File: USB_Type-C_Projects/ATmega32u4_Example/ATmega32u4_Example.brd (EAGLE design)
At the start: 9.2 x 7.2 mm, 52 parts, among them J1 105450-0101, J2 282834-3, J3 282834-3, J4 MF-CON-2.54mm-01x11, J5 MF-CON-2.54mm-01x11, SW1 MF-SW-TACT-4.2MM, SW2 MF-SW-TACT-4.2MM, SW3 MF-SW-TACT-4.2MM, SW4 MF-SW-TACT-4.2MM, SW5 MF-SW-TACT-4.2MM, U1 IP4234CZ6,125, U2 ATMEGA32U4-AU, X1 ABM3B-16.000MHZ-D-1-X-T

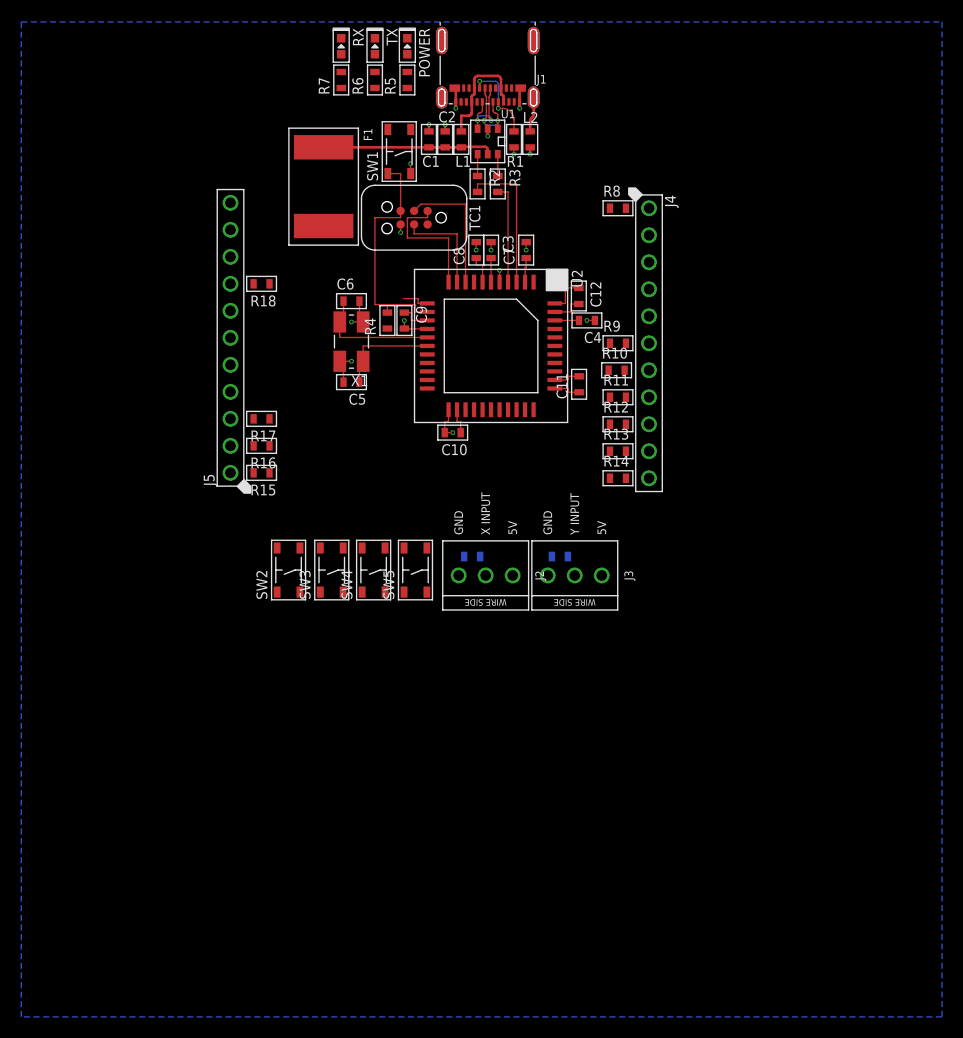
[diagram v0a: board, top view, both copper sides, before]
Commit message: Routing complete
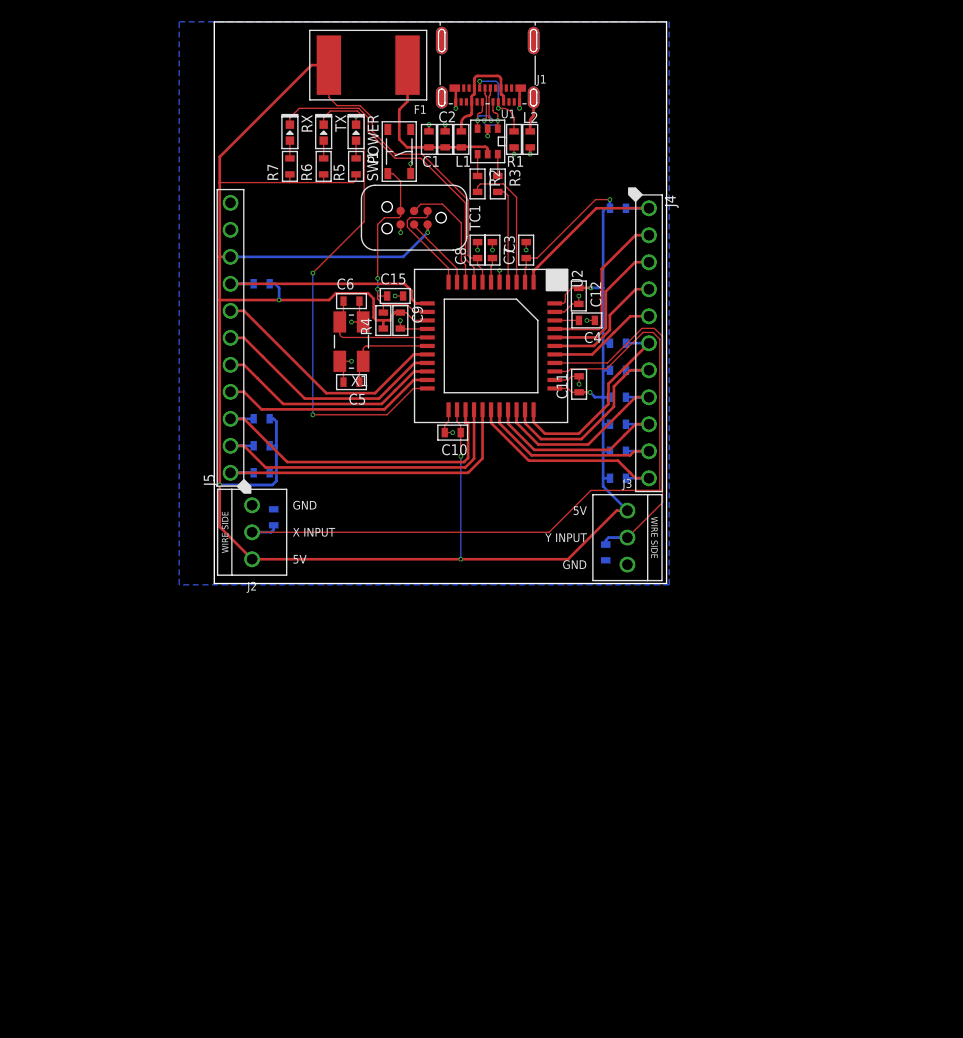
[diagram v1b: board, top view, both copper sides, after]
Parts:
- removed SW2, SW3, SW4, SW5: MF-SW-TACT-4.2MM, MF_Switches:TACT4.2MM
- added C15: 0.1uF, MF_Passives:C0603
- moved J2 22.3 mm to (-7.24, 13.5), turned to 90 degrees
- moved C13 19.0 mm to (-5.21, 14.9), turned to 90 degrees
- moved F1 12.2 mm to (3.68, 57.4), turned to 180 degrees
- moved POWER 9.45 mm to (2.54, 51.1)
- moved R5 9.45 mm to (2.54, 47.9)
- moved R6 9.45 mm to (-0.51, 47.9)
- moved R7 9.45 mm to (-3.68, 47.9)
- moved RX 9.45 mm to (-3.68, 51.1)
- moved TX 9.45 mm to (-0.51, 51.1)
- moved J3 6.10 mm to (28.1, 13.0), turned to 270 degrees
- moved C14 4.33 mm to (26.0, 11.6), turned to 270 degrees
- moved C9 0.38 mm to (6.71, 33.4)
- moved R4 0.38 mm to (5.11, 33.4)
- moved R10 0.13 mm to (27.2, 28.7), flipped to the bottom, turned to 180 degrees
- moved C3 0.13 mm to (15.4, 40.0)
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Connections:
- net 5V: now also R6.P$1, R7.P$1
- net D4: no longer SW2.P$1, SW2.P$2
- net D5*: no longer SW3.P$1, SW3.P$2
- net D6*: no longer SW4.P$1, SW4.P$2
- net D7: no longer SW5.P$1, SW5.P$2
- net GND: now also C15.P$2, J5.P$11; no longer RX.CATHODE, SW2.P$3, SW2.P$4, SW3.P$3, SW3.P$4, SW4.P$3, SW4.P$4, SW5.P$3, SW5.P$4, TX.CATHODE
- net RESET: now also C15.P$1
- net RXLED: now also RX.CATHODE; no longer R7.P$1
- net TXLED: now also TX.CATHODE; no longer R6.P$1
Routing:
- net 5V: track 17.0 -> 267.3 mm, vias 0 -> 8
- net A0: track 0.00 -> 68.4 mm
- net TXLED: track 0.00 -> 46.7 mm, vias 0 -> 2
- net A1: track 0.00 -> 34.6 mm
- net D4: track 0.00 -> 31.1 mm
- net D6*: track 0.00 -> 31.0 mm
- net IO12: track 0.00 -> 30.9 mm
- net RXLED: track 0.00 -> 29.8 mm
- net D3/SCL: track 0.00 -> 23.2 mm
- net D2/SDA: track 0.00 -> 22.3 mm
- net D0/RX: track 0.00 -> 21.3 mm
- net IO8: track 0.00 -> 20.4 mm
- net D1/TX: track 0.00 -> 20.3 mm
- net IO13*: track 0.00 -> 19.5 mm
- net HWB: track 0.00 -> 19.3 mm
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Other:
- board size 9.2 x 7.2 mm -> 42.5 x 52.8 mm

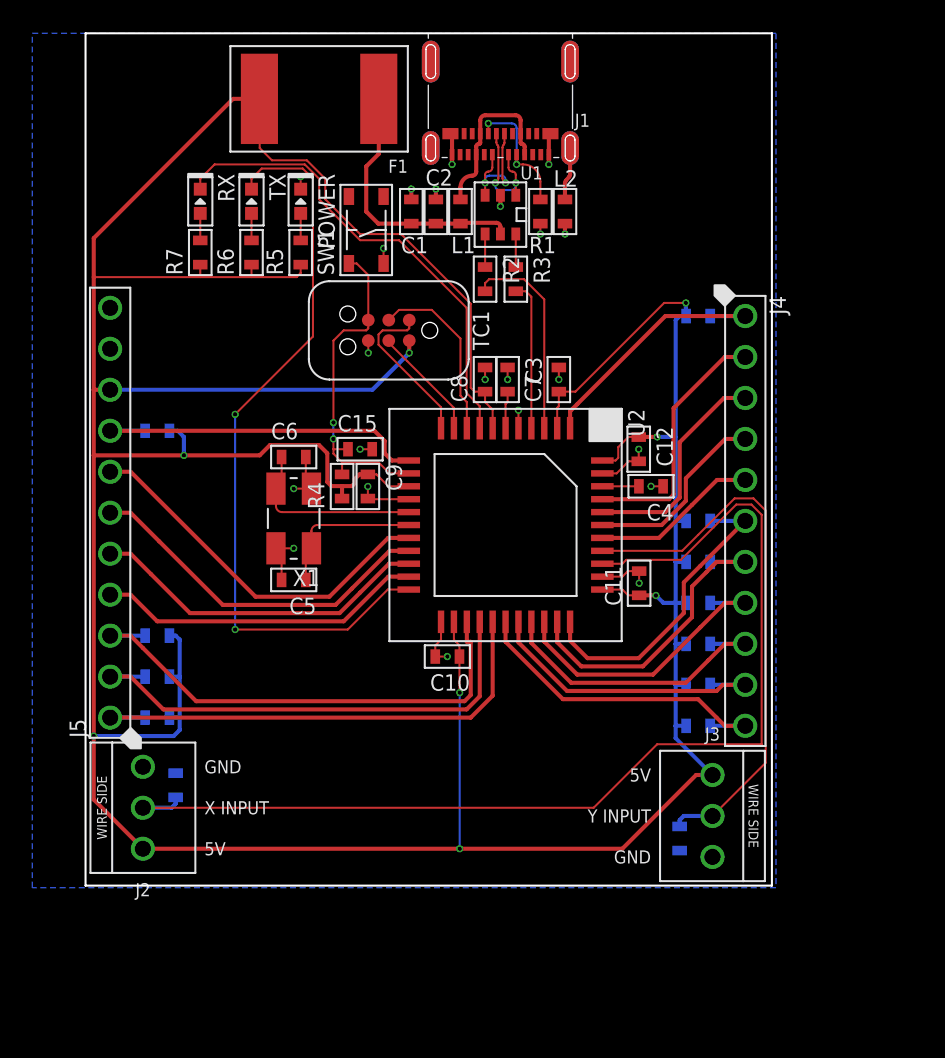
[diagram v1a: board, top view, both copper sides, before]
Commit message: PCB complete. First rev ordered.
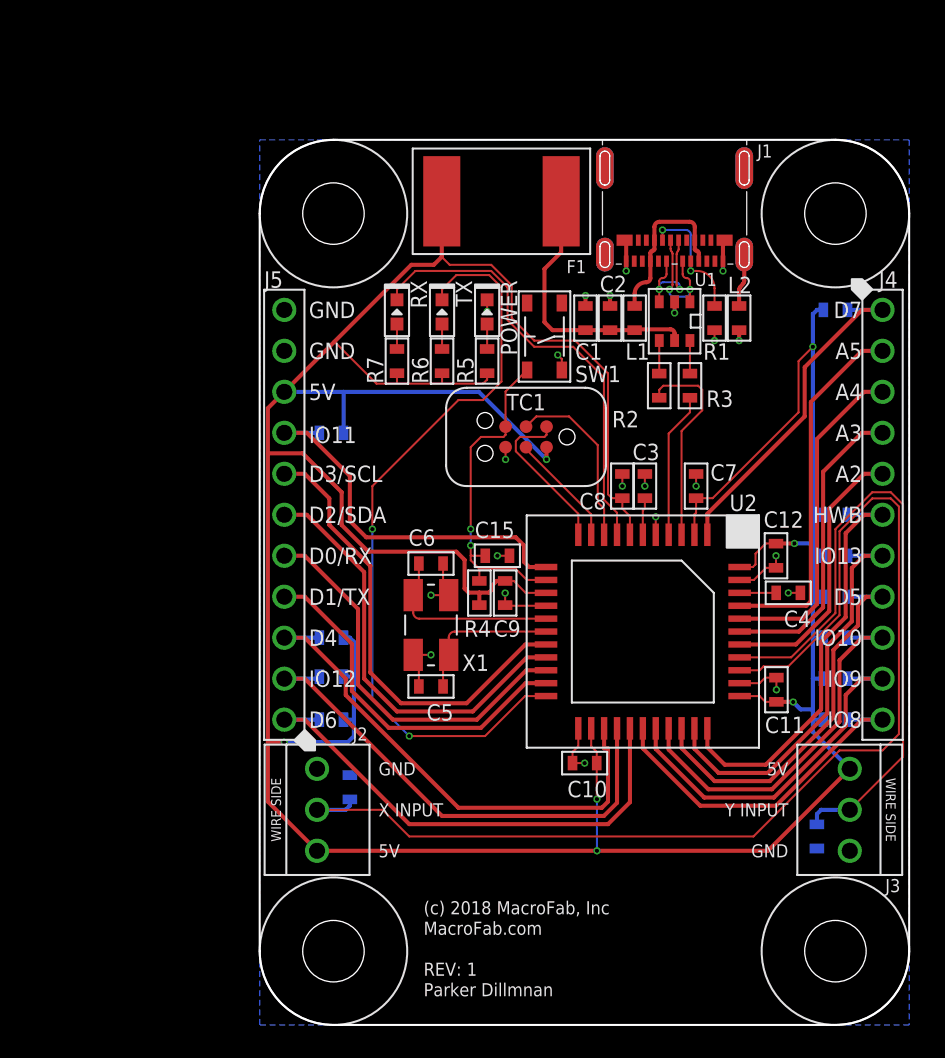
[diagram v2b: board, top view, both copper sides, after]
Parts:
- added FRAME1: MF_FRAMEDEFAULT, MF_Aesthetics:MF_FRAME_DEFAULT
- added H1, H2, H3, H4: MOUNT_HOLE150MIL, PP_Connectors:MOUNT_HOLE_150MIL
- moved RX 14.0 mm to (8.51, 44.2)
- moved R7 13.9 mm to (8.51, 41.1)
- moved TX 13.7 mm to (11.3, 44.2)
- moved R6 13.6 mm to (11.3, 41.1)
- moved POWER 13.4 mm to (14.1, 44.2)
- moved R5 13.4 mm to (14.1, 41.1)
- moved F1 13.0 mm to (15.0, 51.1)
- moved SW1 12.9 mm to (17.7, 42.7)
- moved C1 12.7 mm to (20.2, 43.8)
- moved J1 12.7 mm to (25.7, 47.8)
- moved L1 12.7 mm to (23.2, 43.8)
- moved L2 12.7 mm to (29.7, 43.8)
- moved R2 12.7 mm to (24.8, 39.6)
- moved R3 12.7 mm to (26.7, 39.6)
- moved U1 12.7 mm to (25.7, 43.6)
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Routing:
- net 5V: track 267.3 -> 246.2 mm, vias 8 -> 7
- net HWB: track 19.3 -> 26.6 mm
- net A3: track 11.9 -> 18.9 mm
- net A5: track 15.6 -> 22.6 mm
- net A4: track 13.8 -> 20.7 mm
- net A2: track 10.3 -> 17.0 mm
- net A1: track 34.6 -> 40.8 mm
- net IO13*: track 19.5 -> 25.7 mm
- net D5*: track 18.5 -> 24.6 mm
- net D3/SCL: track 23.2 -> 28.5 mm
- net A0: track 68.4 -> 73.6 mm
- net IO10*: track 18.8 -> 23.9 mm
- net D7: track 16.5 -> 21.4 mm
- net D2/SDA: track 22.3 -> 26.5 mm
- net IO9*: track 18.9 -> 22.9 mm
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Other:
- board size 42.5 x 52.8 mm -> 40.3 x 54.9 mm
